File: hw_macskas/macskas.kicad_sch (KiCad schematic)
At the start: 39 parts, among them J1 Conn_2Rows-05Pins, Q1 AO3401A, Q2 AO3401A, Q3 AO3401A, SW1 SW_DPST_x2, T1 Tab, U1 PY32F002AF15P6TU

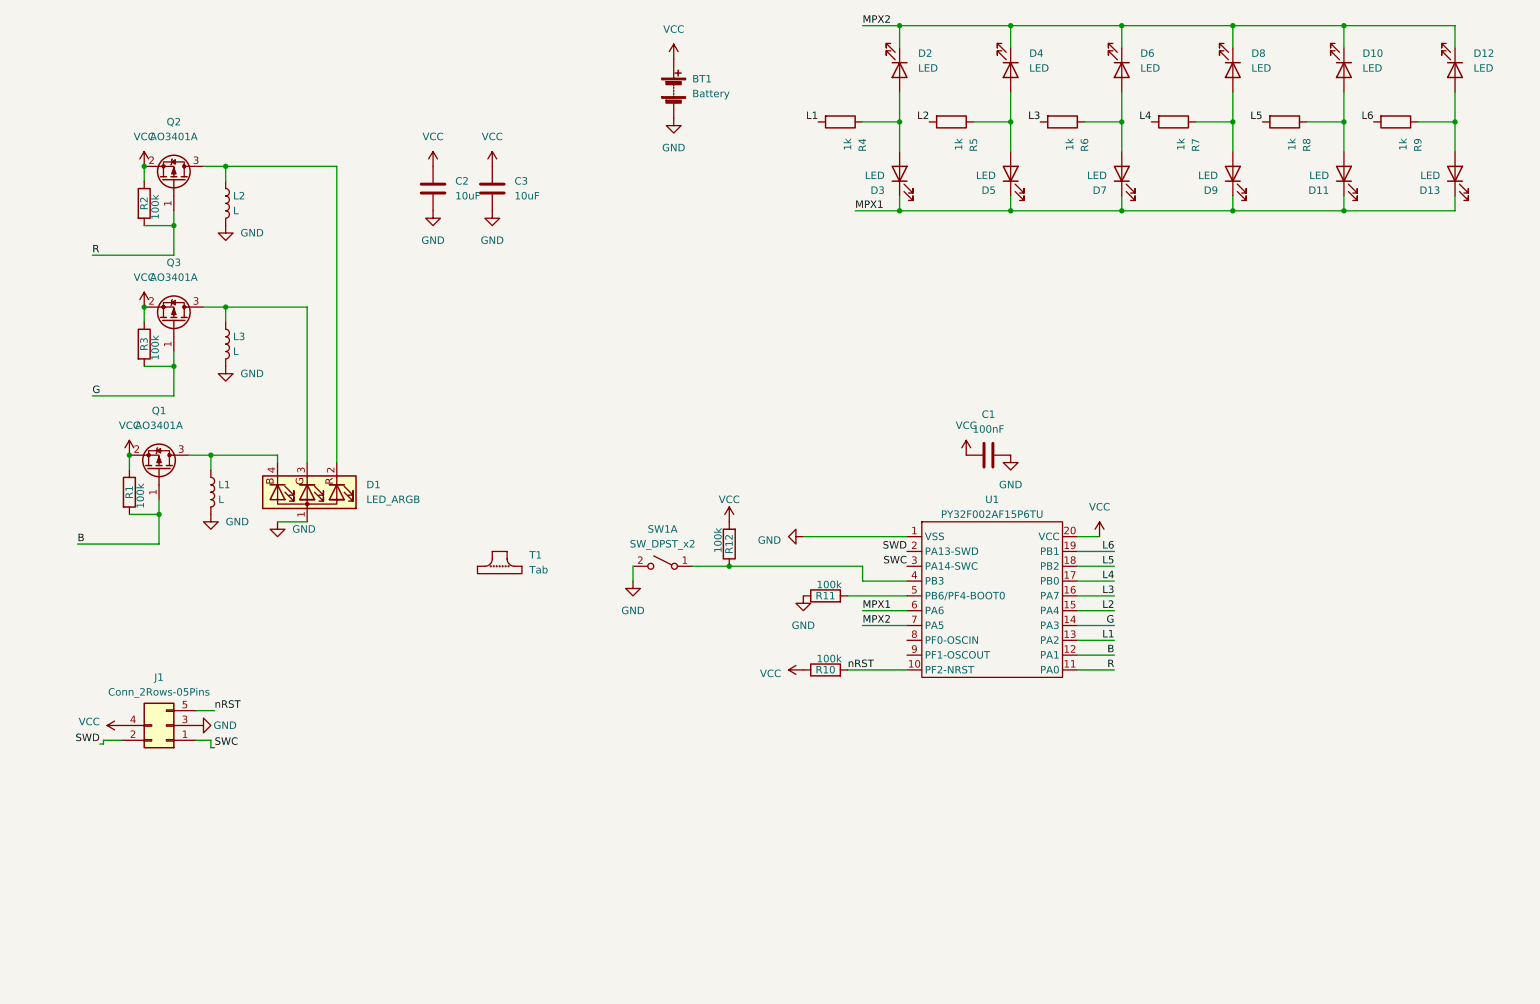
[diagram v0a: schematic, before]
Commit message: Working on cat design.
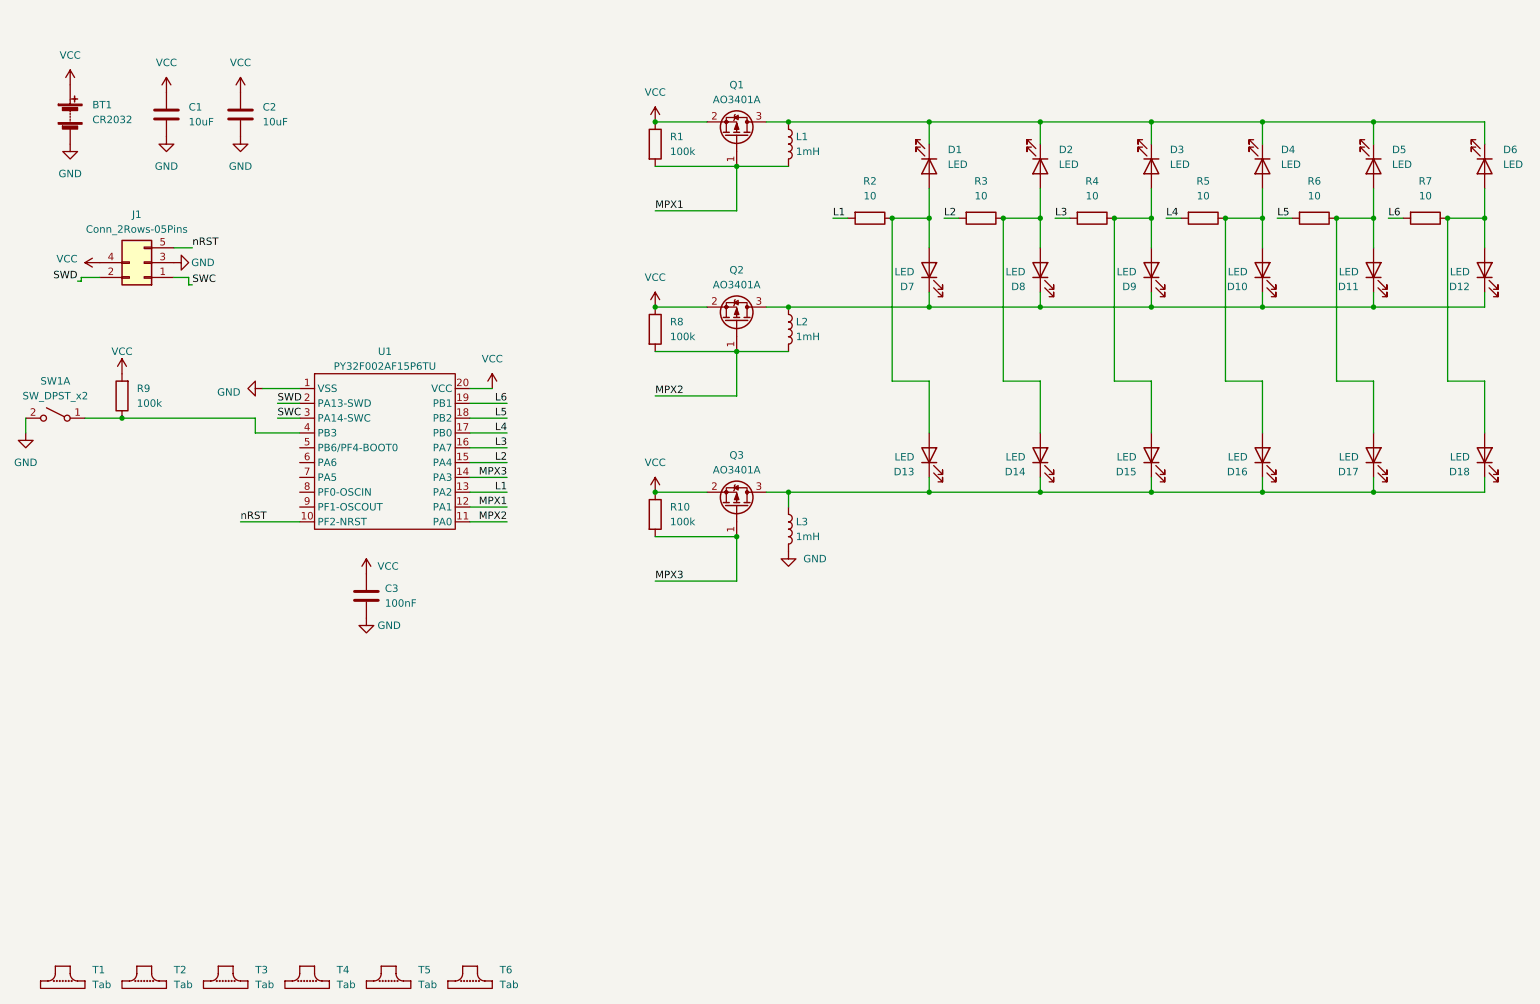
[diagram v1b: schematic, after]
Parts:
- removed D1: LED_ARGB, karifa:LED_RGB_Wuerth-PLCC4_3.2x2.8mm_150141M173100, symbol Device:LED_ARGB
- removed R10, R11: 100k, Resistor_SMD:R_0603_1608Metric, symbol Device:R
- added D13, D14, D15, D16, D17, D18: LED, LED_SMD:LED_0805_2012Metric, symbol Device:LED
- added T2, T3, T4, T5, T6: Tab, kikit:Tab, symbol kikit:Tab
- BT1: value Battery -> CR2032
- L1, L2, L3: value L -> 1mH; footprint Inductor_SMD:L_1008_2520Metric -> Inductor_SMD:L_Ferrocore_DLG-0403
- R2: renamed from R4; value 1k -> 10
- R3: renamed from R5; value 1k -> 10
- R4: renamed from R6; value 1k -> 10
- R5: renamed from R7; value 1k -> 10
- R6: renamed from R8; value 1k -> 10
- R7: renamed from R9; value 1k -> 10
- renumbered C2 to C1, C3 to C2, C1 to C3, D2 to D1, D9 to D10, D13 to D12, D4 to D2, D6 to D3, D8 to D4, D10 to D5, D12 to D6, D3 to D7, D5 to D8, D7 to D9, R3 to R10, R2 to R8, R12 to R9
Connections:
- net B is gone; now on net MPX1: Q1.1 (G), R1.2, U1.12 (PA1)
- net R is gone; now on net MPX2: Q2.1 (G), R8.2, U1.11 (PA0)
- net GND: no longer L1.2, L2.2
- net MPX1: now also L1.2; no longer D10.1 (K), D11.1 (K), D12.1 (K), D7.1 (K), D8.1 (K), D9.1 (K), U1.6 (PA6)
- net MPX2: now also L2.2; no longer D1.1 (K), D2.1 (K), D3.1 (K), D4.1 (K), D5.1 (K), D6.1 (K), U1.7 (PA5)
- net at D11.2 (A), D5.2 (A), R6.1: now also D17.2 (A)
- net at D12.2 (A), D6.2 (A), R7.1: now also D18.2 (A)
- net at L2.1, Q2.3 (D): now also D10.1 (K), D11.1 (K), D12.1 (K), D7.1 (K), D8.1 (K), D9.1 (K)
- net at D3.2 (A), D9.2 (A), R4.1: now also D15.2 (A)
- net at L3.1, Q3.3 (D): now also D13.1 (K), D14.1 (K), D15.1 (K), D16.1 (K), D17.1 (K), D18.1 (K)
- net at D1.2 (A), D7.2 (A), R2.1: now also D13.2 (A)
- net at D2.2 (A), D8.2 (A), R3.1: now also D14.2 (A)
- net at D10.2 (A), D4.2 (A), R5.1: now also D16.2 (A)
- net at L1.1, Q1.3 (D): now also D1.1 (K), D2.1 (K), D3.1 (K), D4.1 (K), D5.1 (K), D6.1 (K)
- net G renamed MPX3
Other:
- moved on the sheet: BT1, C1, C2, C3, D1, D10, D11, D12, D2, D3, D4, D5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

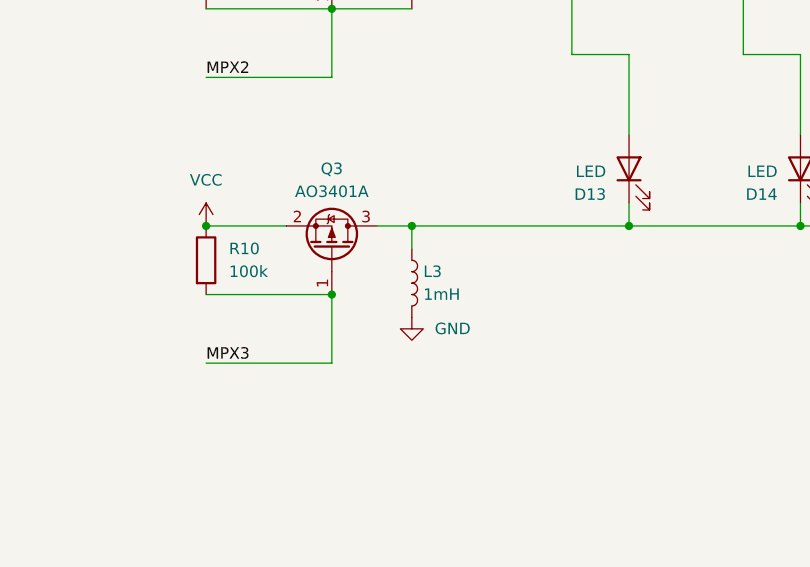
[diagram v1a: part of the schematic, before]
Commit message: Updated cat.
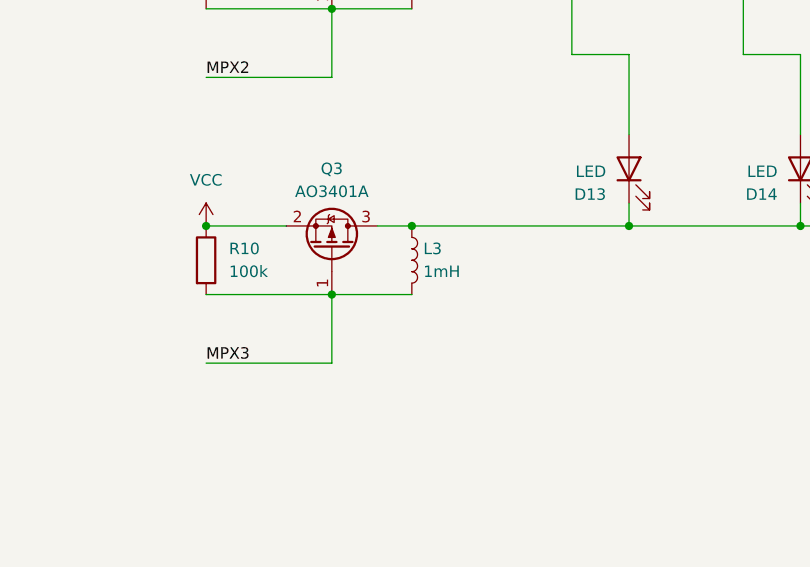
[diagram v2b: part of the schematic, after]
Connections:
- net GND: no longer L3.2
- net MPX3: now also L3.2
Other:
- moved on the sheet: L3
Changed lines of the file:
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@@
 	(wire
 		(pts
-			(xy 149.86 101.6) (xy 149.86 104.14)
-		)
-		(stroke
-			(width 0)
-			(type default)
-		)
-	)
-	(wire
-		(pts
 			(xy 127 109.22) (xy 140.97 109.22)
 		)
@@
 	(wire
 		(pts
-			(xy 140.97 109.22) (xy 140.97 116.84)
-		)
-		(stroke
-			(width 0)
-			(type default)
-		)
-	)
-	(wire
-		(pts
 			(xy 269.24 99.06) (xy 269.24 101.6)
 		)
@@
 	(wire
 		(pts
+			(xy 140.97 109.22) (xy 149.86 109.22)
+		)
+		(stroke
+			(width 0)
+			(type default)
+		)
+	)
+	(wire
+		(pts
 			(xy 193.04 69.85) (xy 212.09 69.85)
 		)
@@
 	(wire
 		(pts
+			(xy 140.97 109.22) (xy 140.97 116.84)
+		)
+		(stroke
+			(width 0)
+			(type default)
+		)
+	)
+	(wire
+		(pts
 			(xy 193.04 91.44) (xy 193.04 82.55)
 		)
@@
 	(symbol
 		(lib_id "Device:L")
-		(at 149.86 107.95 0)
+		(at 149.86 105.41 0)
 		(unit 1)
 		(exclude_from_sim no)
@@
 		(fields_autoplaced yes)
 		(property "Reference" "L3"
-			(at 151.13 106.6799 0)
+			(at 151.13 104.1399 0)
 			(effects
 				(font
@@
 		)
 		(property "Value" "1mH"
-			(at 151.13 109.2199 0)
+			(at 151.13 106.6799 0)
 			(effects
 				(font
@@
 		)
 		(property "Footprint" "Inductor_SMD:L_Ferrocore_DLG-0403"
-			(at 149.86 107.95 0)
+			(at 149.86 105.41 0)
 			(effects
 				(font
@@
 		)
 		(property "Datasheet" "~"
-			(at 149.86 107.95 0)
+			(at 149.86 105.41 0)
 			(effects
 				(font
@@
 		)
 		(property "Description" ""
-			(at 149.86 107.95 0)
+			(at 149.86 105.41 0)
 			(effects
 				(font
@@
 					(unit 1)
 				)
-			)
-		)
-	)
-	(symbol
-		(lib_id "power:GND")
-		(at 149.86 111.76 0)
-		(unit 1)
-		(exclude_from_sim no)
-		(in_bom yes)
-		(on_board yes)
-		(dnp no)
-		(fields_autoplaced yes)
-		(property "Reference" "#PWR016"
-			(at 149.86 118.11 0)
-			(effects
-				(font
-					(size 1.27 1.27)
-				)
-				(hide yes)
-			)
-		)
-		(property "Value" "GND"
-			(at 152.4 113.0299 0)
-			(effects
-				(font
-					(size 1.27 1.27)
-				)
-				(justify left)
-			)
-		)
-		(property "Footprint" ""
-			(at 149.86 111.76 0)
-			(effects
-				(font
-					(size 1.27 1.27)
-				)
-				(hide yes)
-			)
-		)
-		(property "Datasheet" ""
-			(at 149.86 111.76 0)
-			(effects
-				(font
-					(size 1.27 1.27)
-				)
-				(hide yes)
-			)
-		)
-		(property "Description" ""
-			(at 149.86 111.76 0)
-			(effects
-				(font
-					(size 1.27 1.27)
-				)
-				(hide yes)
-			)
-		)
-		(pin "1"
-		)
-		(instances
-			(project "hopehely"
-				(path "/30f28fd8-ef05-4208-b612-7ffefcdba2ba"
-					(reference "#PWR016")
-					(unit 1)
-				)
